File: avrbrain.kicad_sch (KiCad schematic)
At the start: 46 parts, among them J1 XKTF-0803-0, J12 PD/PE, J2 U254-051T-4BH81-S2S, J4 UPDI, J5 UEXT, J6 PC, J7 PA/PB, J8 PG, J9 SM04B-SRSS-TB, Q1 BSS138, SW1 RESET, SW2 VDD, U1 CH340C, U2 AVR128DB64x-xPT, U3 PCF8563T, U5 AMS1117-3.3, Y1 32kHz

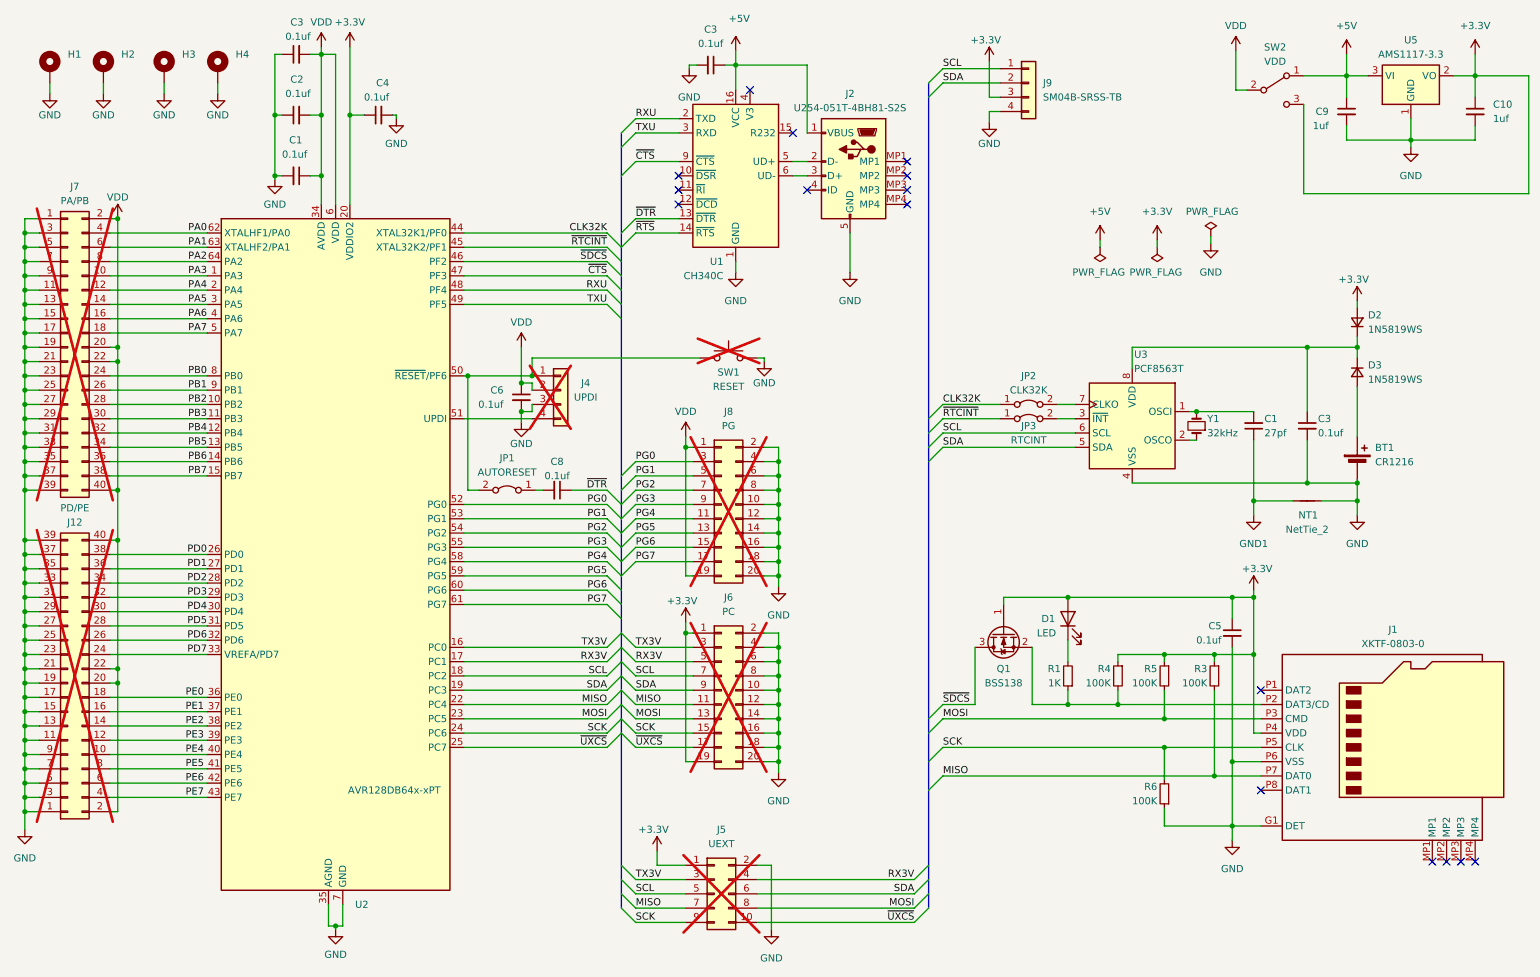
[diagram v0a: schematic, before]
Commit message: Finish layout and routing
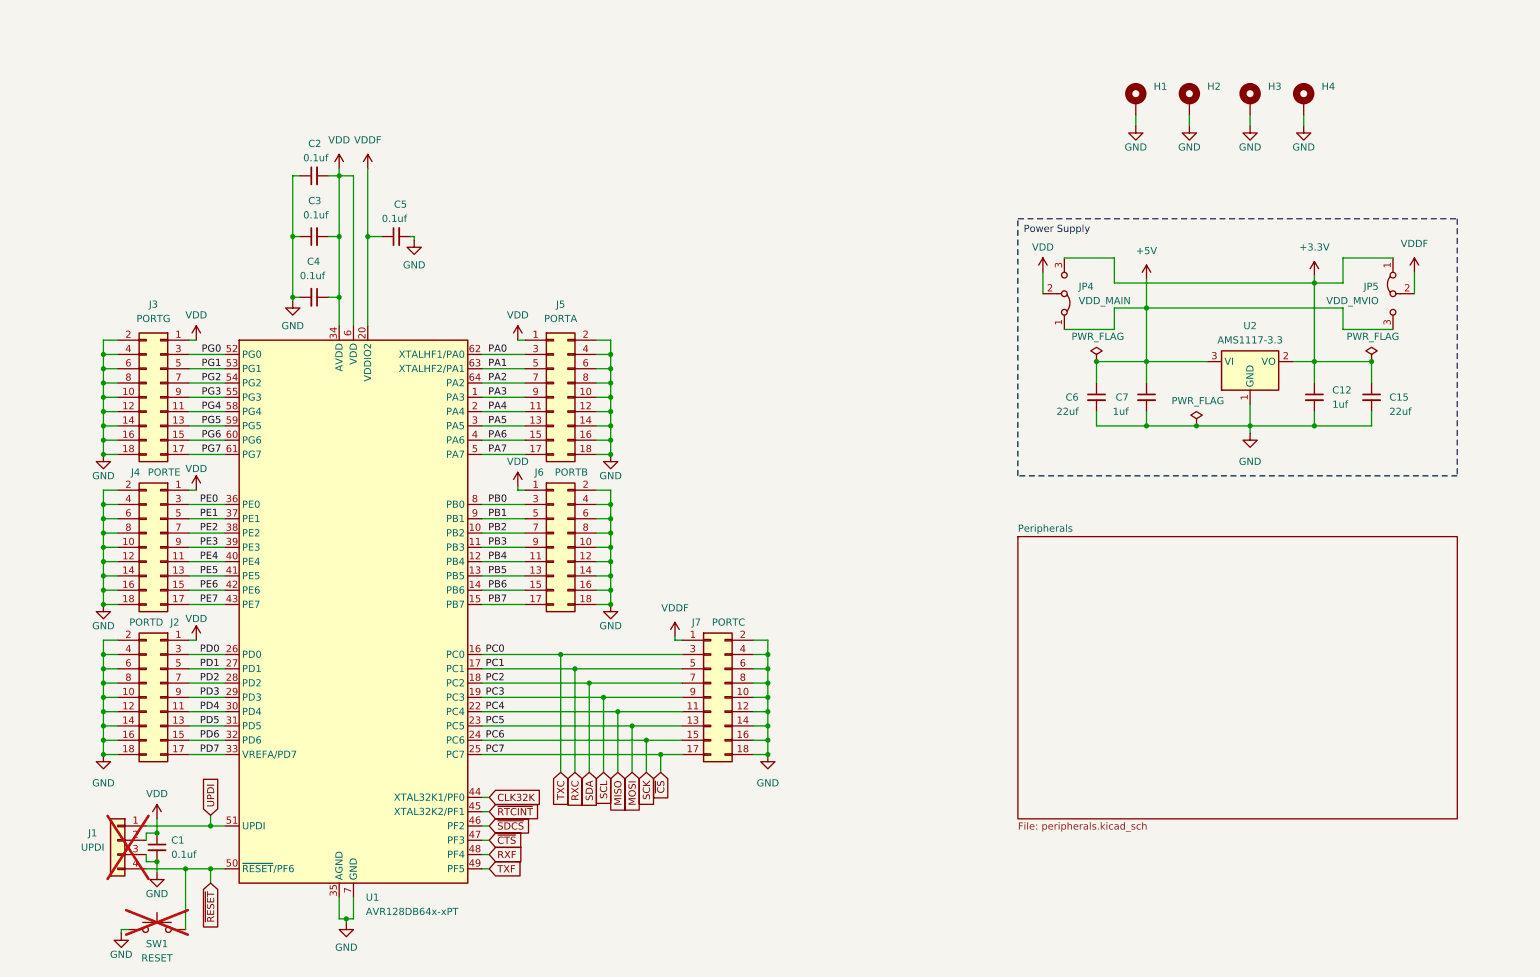
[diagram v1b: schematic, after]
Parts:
- removed BT1: CR1216, Battery:BatteryHolder_Keystone_3001_1x12mm, symbol Device:Battery_Cell
- removed C1: 27pf, Capacitor_SMD:C_0603_1608Metric, symbol Device:C_Small
- removed C10, C9: 1uf, Capacitor_SMD:C_1206_3216Metric, symbol Device:C_Small
- removed C3 (x2), C5, C8: 0.1uf, Capacitor_SMD:C_0402_1005Metric, symbol Device:C_Small
- removed D1: LED, LED_SMD:LED_0805_2012Metric, symbol Device:LED
- removed D2, D3: 1N5819WS, Diode_SMD:D_SOD-323_HandSoldering, symbol Device:D_Small
- removed J1: XKTF-0803-0, SamacSys_Parts:XKTF08030, symbol Connector:Micro_SD_Card_Det1
- removed J12: PD/PE, Connector_PinHeader_2.54mm:PinHeader_2x20_P2.54mm_Vertical, symbol Connector_Generic:Conn_02x20_Odd_Even
- removed J2: U254-051T-4BH81-S2S, SamacSys_Parts:U254051T4BH81S2S, symbol Connector:USB_B_Micro
- removed J5: UEXT, Connector_IDC:IDC-Header_2x05_P2.54mm_Horizontal, symbol Connector_Generic:Conn_02x05_Odd_Even
- removed J6: PC, Connector_PinHeader_2.54mm:PinHeader_2x10_P2.54mm_Vertical, symbol Connector_Generic:Conn_02x10_Odd_Even
- removed J7: PA/PB, Connector_PinHeader_2.54mm:PinHeader_2x20_P2.54mm_Vertical, symbol Connector_Generic:Conn_02x20_Odd_Even
- removed J8: PG, Connector_PinHeader_2.54mm:PinHeader_2x10_P2.54mm_Vertical, symbol Connector_Generic:Conn_02x10_Odd_Even
- removed J9: SM04B-SRSS-TB, Custom:JST_SM04B-SRSS-TB_LF__SN_, symbol Connector_Generic:Conn_01x04
- removed JP1: AUTORESET, Jumper:SolderJumper-2_P1.3mm_Bridged_Pad1.0x1.5mm, symbol Jumper:Jumper_2_Bridged
- removed JP2: CLK32K, Jumper:SolderJumper-2_P1.3mm_Bridged_Pad1.0x1.5mm, symbol Jumper:Jumper_2_Bridged
- removed JP3: RTCINT, Jumper:SolderJumper-2_P1.3mm_Bridged_Pad1.0x1.5mm, symbol Jumper:Jumper_2_Bridged
- removed NT1: NetTie_2, NetTie:NetTie-2_SMD_Pad0.5mm, symbol Device:NetTie_2
- removed Q1: BSS138, Package_TO_SOT_SMD:SOT-23, symbol Transistor_FET:BSS138
- removed R1: 1K, Resistor_SMD:R_0402_1005Metric, symbol Device:R_Small
- removed R3, R4, R5, R6: 100K, Resistor_SMD:R_0402_1005Metric, symbol Device:R_Small
- removed SW2: VDD, SamacSys_Parts:JS202011CQN, symbol Switch:SW_SPDT
- removed U1: CH340C, Package_SO:SOIC-16_3.9x9.9mm_P1.27mm, symbol Interface_USB:CH340C
- removed U2: AVR128DB64x-xPT, Package_QFP:TQFP-64_10x10mm_P0.5mm, symbol MCU_Microchip_AVR_Dx:AVR128DB64x-xPT
- removed U3: PCF8563T, Package_SO:SOIC-8_3.9x4.9mm_P1.27mm, symbol Timer_RTC:PCF8563T
- removed U5: AMS1117-3.3, Package_TO_SOT_SMD:SOT-223-3_TabPin2, symbol Regulator_Linear:AMS1117-3.3
- removed Y1: 32kHz, Crystal:Crystal_SMD_3215-2Pin_3.2x1.5mm, symbol Device:Crystal_Small
- added C12, C7: 1uf, Capacitor_SMD:C_1206_3216Metric, symbol Device:C_Small
- added C15, C6: 22uf, Capacitor_SMD:C_1206_3216Metric, symbol Device:C_Small
- added J2: PORTD, Connector_PinSocket_2.54mm:PinSocket_2x09_P2.54mm_Vertical, symbol Connector_Generic:Conn_02x09_Odd_Even
- added J3: PORTG, Connector_PinSocket_2.54mm:PinSocket_2x09_P2.54mm_Vertical, symbol Connector_Generic:Conn_02x09_Odd_Even
- added J4: PORTE, Connector_PinSocket_2.54mm:PinSocket_2x09_P2.54mm_Vertical, symbol Connector_Generic:Conn_02x09_Odd_Even
- added J5: PORTA, Connector_PinSocket_2.54mm:PinSocket_2x09_P2.54mm_Vertical, symbol Connector_Generic:Conn_02x09_Odd_Even
- added J6: PORTB, Connector_PinSocket_2.54mm:PinSocket_2x09_P2.54mm_Vertical, symbol Connector_Generic:Conn_02x09_Odd_Even
- added J7: PORTC, Connector_PinSocket_2.54mm:PinSocket_2x09_P2.54mm_Vertical, symbol Connector_Generic:Conn_02x09_Odd_Even
- added JP4: VDD_MAIN, Jumper:SolderJumper-3_P1.3mm_Bridged2Bar12_RoundedPad1.0x1.5mm, symbol Jumper:Jumper_3_Bridged12
- added JP5: VDD_MVIO, Jumper:SolderJumper-3_P1.3mm_Bridged2Bar12_RoundedPad1.0x1.5mm, symbol Jumper:Jumper_3_Bridged12
- added U1: AVR128DB64x-xPT, Package_QFP:TQFP-64_10x10mm_P0.5mm, symbol MCU_Microchip_AVR_Dx:AVR128DB64x-xPT
- added U2: AMS1117-3.3, Package_TO_SOT_SMD:SOT-223-3_TabPin2, symbol Regulator_Linear:AMS1117-3.3
- renumbered C6 to C1, C3 to C2, C2 to C3, C1 to C4, C4 to C5, J4 to J1
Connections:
- net +3.3V: now also C12.1, C15.1, JP4.3 (B), JP5.1 (A), U2.2 (VO); no longer C5.1
- net +5V: now also C6.1, C7.1, JP4.1 (A), JP5.3 (B), U2.3 (VI)
- net CLK32K: now also U1.44 (XTAL32K1/PF0)
- net GND: now also C12.2, C15.2, C6.2, C7.2, J2.10 (Pin_10), J2.12 (Pin_12), J2.14 (Pin_14), J2.16 (Pin_16), J2.18 (Pin_18), J2.2 (Pin_2), J2.4 (Pin_4), J2.6 (Pin_6), J2.8 (Pin_8), J3.10 (Pin_10), J3.12 (Pin_12), J3.14 (Pin_14), J3.16 (Pin_16), J3.18 (Pin_18), J3.2 (Pin_2), J3.4 (Pin_4), J3.6 (Pin_6), J3.8 (Pin_8), J4.10 (Pin_10), J4.12 (Pin_12), J4.14 (Pin_14), J4.16 (Pin_16), J4.18 (Pin_18), J4.2 (Pin_2), J4.4 (Pin_4), J4.6 (Pin_6), J4.8 (Pin_8), J5.10 (Pin_10), J5.12 (Pin_12), J5.14 (Pin_14), J5.16 (Pin_16), J5.18 (Pin_18), J5.2 (Pin_2), J5.4 (Pin_4), J5.6 (Pin_6), J5.8 (Pin_8), J6.10 (Pin_10), J6.12 (Pin_12), J6.14 (Pin_14), J6.16 (Pin_16), J6.18 (Pin_18), J6.2 (Pin_2), J6.4 (Pin_4), J6.6 (Pin_6), J6.8 (Pin_8), J7.10 (Pin_10), J7.12 (Pin_12), J7.14 (Pin_14), J7.16 (Pin_16), J7.18 (Pin_18), J7.2 (Pin_2), J7.4 (Pin_4), J7.6 (Pin_6), J7.8 (Pin_8), U1.21 (GND), U1.35 (AGND), U1.57 (GND), U1.7 (GND), U2.1 (GND)
- net MISO: now also J7.11 (Pin_11), U1.22 (PC4)
- net MOSI: now also J7.13 (Pin_13), U1.23 (PC5)
- net PA0: now also J5.3 (Pin_3), U1.62 (XTALHF1/PA0)
- net PA1: now also J5.5 (Pin_5), U1.63 (XTALHF2/PA1)
- net PA2: now also J5.7 (Pin_7), U1.64 (PA2)
- net PA3: now also J5.9 (Pin_9), U1.1 (PA3)
- net PA4: now also J5.11 (Pin_11), U1.2 (PA4)
- net PA5: now also J5.13 (Pin_13), U1.3 (PA5)
- net PA6: now also J5.15 (Pin_15), U1.4 (PA6)
- net PA7: now also J5.17 (Pin_17), U1.5 (PA7)
- net PB0: now also J6.3 (Pin_3), U1.8 (PB0)
- net PB1: now also J6.5 (Pin_5), U1.9 (PB1)
- net PB2: now also J6.7 (Pin_7), U1.10 (PB2)
- net PB3: now also J6.9 (Pin_9), U1.11 (PB3)
- net PB4: now also J6.11 (Pin_11), U1.12 (PB4)
- net PB5: now also J6.13 (Pin_13), U1.13 (PB5)
- net PB6: now also J6.15 (Pin_15), U1.14 (PB6)
- net PB7: now also J6.17 (Pin_17), U1.15 (PB7)
- net PD0: now also J2.3 (Pin_3), U1.26 (PD0)
- net PD1: now also J2.5 (Pin_5), U1.27 (PD1)
- net PD2: now also J2.7 (Pin_7), U1.28 (PD2)
- net PD3: now also J2.9 (Pin_9), U1.29 (PD3)
- net PD4: now also J2.11 (Pin_11), U1.30 (PD4)
- net PD5: now also J2.13 (Pin_13), U1.31 (PD5)
- net PD6: now also J2.15 (Pin_15), U1.32 (PD6)
- net PD7: now also J2.17 (Pin_17), U1.33 (VREFA/PD7)
- net PE0: now also J4.3 (Pin_3), U1.36 (PE0)
- net PE1: now also J4.5 (Pin_5), U1.37 (PE1)
- net PE2: now also J4.7 (Pin_7), U1.38 (PE2)
- net PE3: now also J4.9 (Pin_9), U1.39 (PE3)
- net PE4: now also J4.11 (Pin_11), U1.40 (PE4)
- net PE5: now also J4.13 (Pin_13), U1.41 (PE5)
- net PE6: now also J4.15 (Pin_15), U1.42 (PE6)
- net PE7: now also J4.17 (Pin_17), U1.43 (PE7)
- net PG0: now also J3.3 (Pin_3), U1.52 (PG0)
- net PG1: now also J3.5 (Pin_5), U1.53 (PG1)
- net PG2: now also J3.7 (Pin_7), U1.54 (PG2)
- net PG3: now also J3.9 (Pin_9), U1.55 (PG3)
- net PG4: now also J3.11 (Pin_11), U1.58 (PG4)
- net PG5: now also J3.13 (Pin_13), U1.59 (PG5)
- net PG6: now also J3.15 (Pin_15), U1.60 (PG6)
- net PG7: now also J3.17 (Pin_17), U1.61 (PG7)
- net SCK: now also J7.15 (Pin_15), U1.24 (PC6)
- net SCL: now also J7.9 (Pin_9), U1.19 (PC3)
- net SDA: now also J7.7 (Pin_7), U1.18 (PC2)
- net VDD: now also J2.1 (Pin_1), J3.1 (Pin_1), J4.1 (Pin_1), J5.1 (Pin_1), J6.1 (Pin_1), JP4.2 (C), U1.34 (AVDD), U1.56 (VDD), U1.6 (VDD)
- net ~{CTS}: now also U1.47 (PF3)
- net ~{RTCINT}: now also U1.45 (XTAL32K2/PF1)
- net ~{SDCS}: now also U1.46 (PF2)
- net UPDI: now reaches J1.1 (Pin_1)
- net UPDI: now also U1.51 (UPDI); no longer SW1.2
- net ~{RESET}: now reaches J1.4 (Pin_4)
- net ~{RESET}: now also SW1.2, U1.50 (~{RESET}/PF6)
- new net RXC: J7.5 (Pin_5), U1.17 (PC1)
- new net RXF: U1.48 (PF4)
- new net TXC: J7.3 (Pin_3), U1.16 (PC0)
- new net TXF: U1.49 (PF5)
- new net VDDF: C5.1, J7.1 (Pin_1), JP5.2 (C), U1.20 (VDDIO2)
- new net ~{CS}: J7.17 (Pin_17), U1.25 (PC7)
- no-connect marks 16 -> 0
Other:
- added sheet Peripherals (peripherals.kicad_sch)
- title: z80ctrl NG -> AVRbrain
- moved on the sheet: C1, C2, C3, C4, C5, H1, H2, H3, H4, J1, SW1
